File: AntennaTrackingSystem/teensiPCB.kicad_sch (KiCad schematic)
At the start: 11 parts, among them J4 screw terminal, J5 UART1, J6 UART2, J7 I2C ext, SW1 SW_Push, U1 Teensy4.1, U2 SAM-M10Q-00B

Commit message: cleanup
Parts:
- J5, J6, J7: footprint Connector_JST:JST_EH_B4B-EH-A_1x04_P2.50mm_Vertical -> Connector_JST:JST_XH_B4B-XH-A_1x04_P2.50mm_Vertical
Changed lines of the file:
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@@
 			)
 		)
-		(property "Footprint" "Connector_JST:JST_EH_B4B-EH-A_1x04_P2.50mm_Vertical"
+		(property "Footprint" "Connector_JST:JST_XH_B4B-XH-A_1x04_P2.50mm_Vertical"
 			(at 78.74 96.52 0)
 			(effects
@@
 			)
 		)
-		(property "Footprint" "Connector_JST:JST_EH_B4B-EH-A_1x04_P2.50mm_Vertical"
+		(property "Footprint" "Connector_JST:JST_XH_B4B-XH-A_1x04_P2.50mm_Vertical"
 			(at 78.74 78.74 0)
 			(effects
@@
 			)
 		)
-		(property "Footprint" "Connector_JST:JST_EH_B4B-EH-A_1x04_P2.50mm_Vertical"
+		(property "Footprint" "Connector_JST:JST_XH_B4B-XH-A_1x04_P2.50mm_Vertical"
 			(at 78.74 60.96 0)
 			(effects

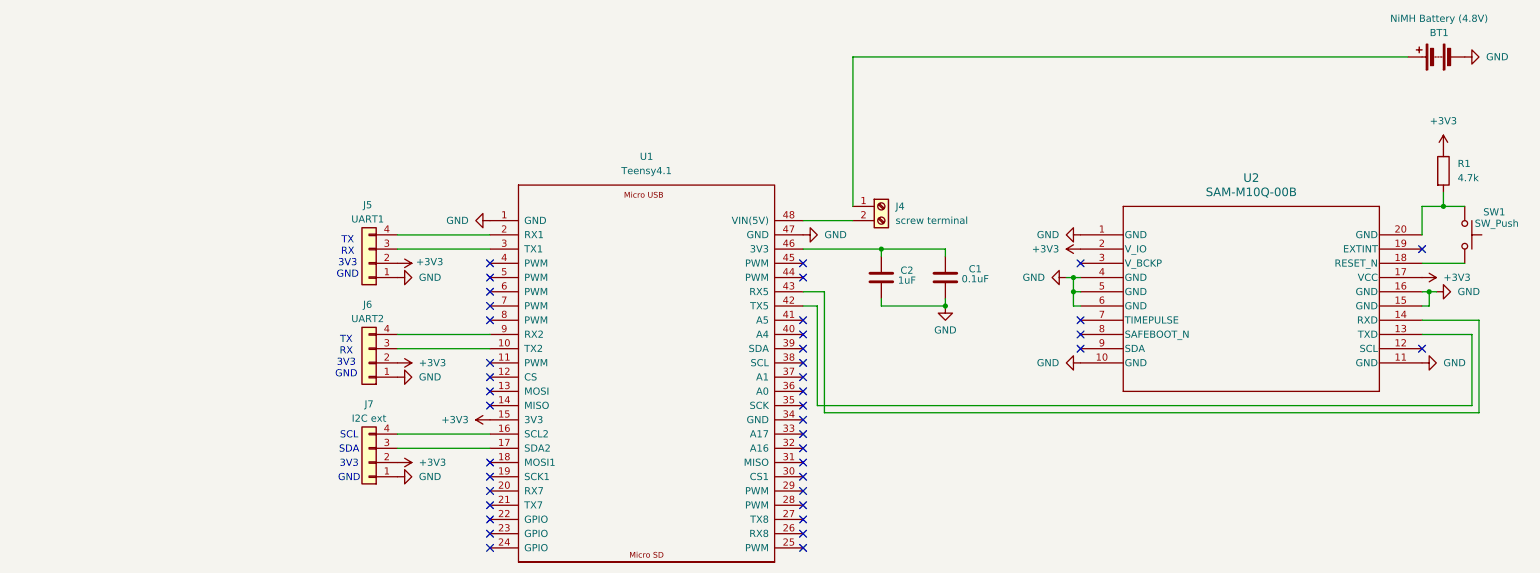
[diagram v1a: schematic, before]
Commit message: back to I2C and other small updates
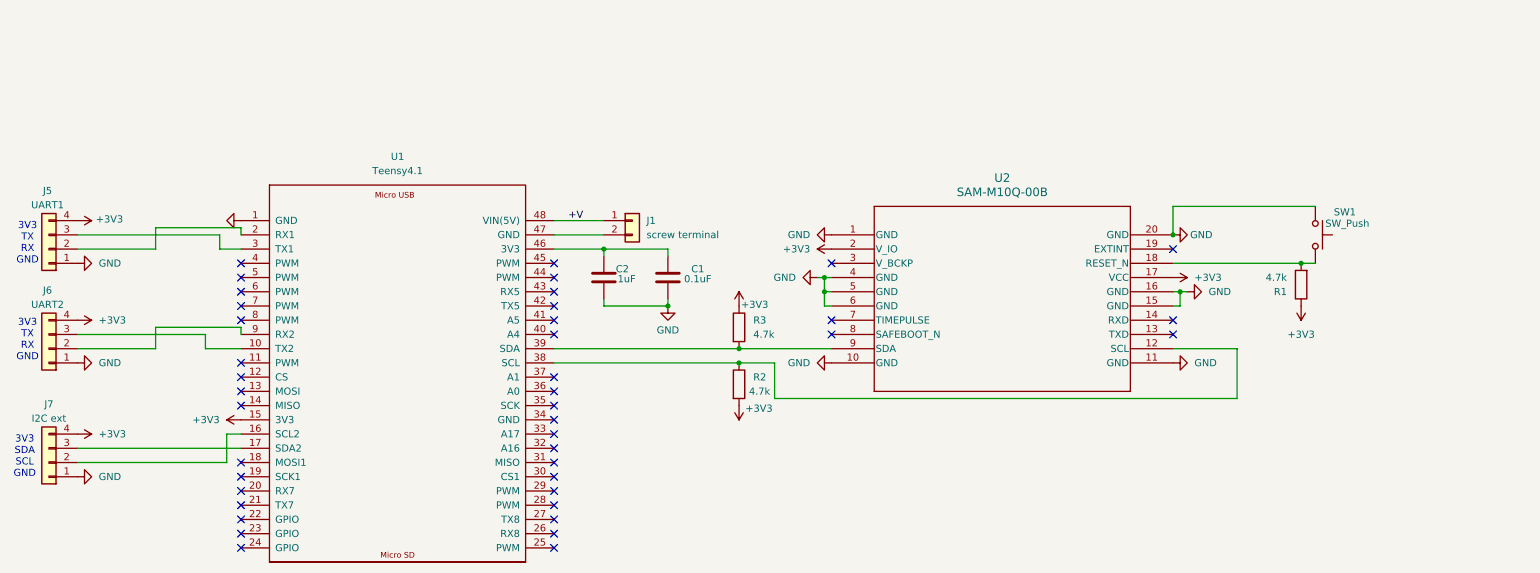
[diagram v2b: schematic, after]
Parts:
- removed BT1: NiMH Battery (4.8V), Battery:BatteryHolder_Keystone_2462_2xAA, symbol Device:Battery
- removed J4: screw terminal, TerminalBlock_MetzConnect:TerminalBlock_MetzConnect_Type073_RT02602HBLU_1x02_P5.08mm_Horizontal, symbol Connector:Screw_Terminal_01x02
- added J1: screw terminal, Connector_JST:JST_XH_B2B-XH-A_1x02_P2.50mm_Vertical, symbol Connector_Generic:Conn_01x02
- added R2, R3: 4.7k, Resistor_SMD:R_0603_1608Metric, symbol Device:R
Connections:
- net +3V3: now also J5.4 (Pin_4), J6.4 (Pin_4), J7.4 (Pin_4), R2.2, R3.1; no longer J5.2 (Pin_2), J6.2 (Pin_2), J7.2 (Pin_2)
- net GND: now also SW1.1, U2.20 (GND); no longer U1.47 (GND)
- net at U1.16 (SCL2): now also J7.2 (Pin_2); no longer J7.4 (Pin_4)
- net at U1.9 (RX2): now also J6.2 (Pin_2); no longer J6.4 (Pin_4)
- net at U1.2 (RX1): now also J5.2 (Pin_2); no longer J5.4 (Pin_4)
- net at U1.38 (SCL): now also U2.12 (SCL), R2.1
- net at U1.39 (SDA): now also U2.9 (SDA), R3.2
- net at U1.42 (TX5): no longer U2.13 (TXD)
- net at U1.43 (RX5): no longer U2.14 (RXD)
- net +V: now reaches U1.48 (VIN(5V))
- net +V: now also J1.1 (Pin_1)
- net at SW1.2, U2.18 (RESET_N): now also R1.2
- new net: J1.2 (Pin_2), U1.47 (GND)
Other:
- note added: "3V3 SDA SCL GND"
- note added: "3V3 TX RX GND"
- note removed: "3V3"
- note removed: "GND"
- note removed: "SCL"
- note removed: "SDA"
- note removed: "TX RX 3V3 GND"
- moved on the sheet: C1, C2, J5, J6, J7, R1, SW1, U1, U2
